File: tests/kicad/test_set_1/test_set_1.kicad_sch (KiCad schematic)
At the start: 46 parts, among them J4 Conn_01x24_Socket

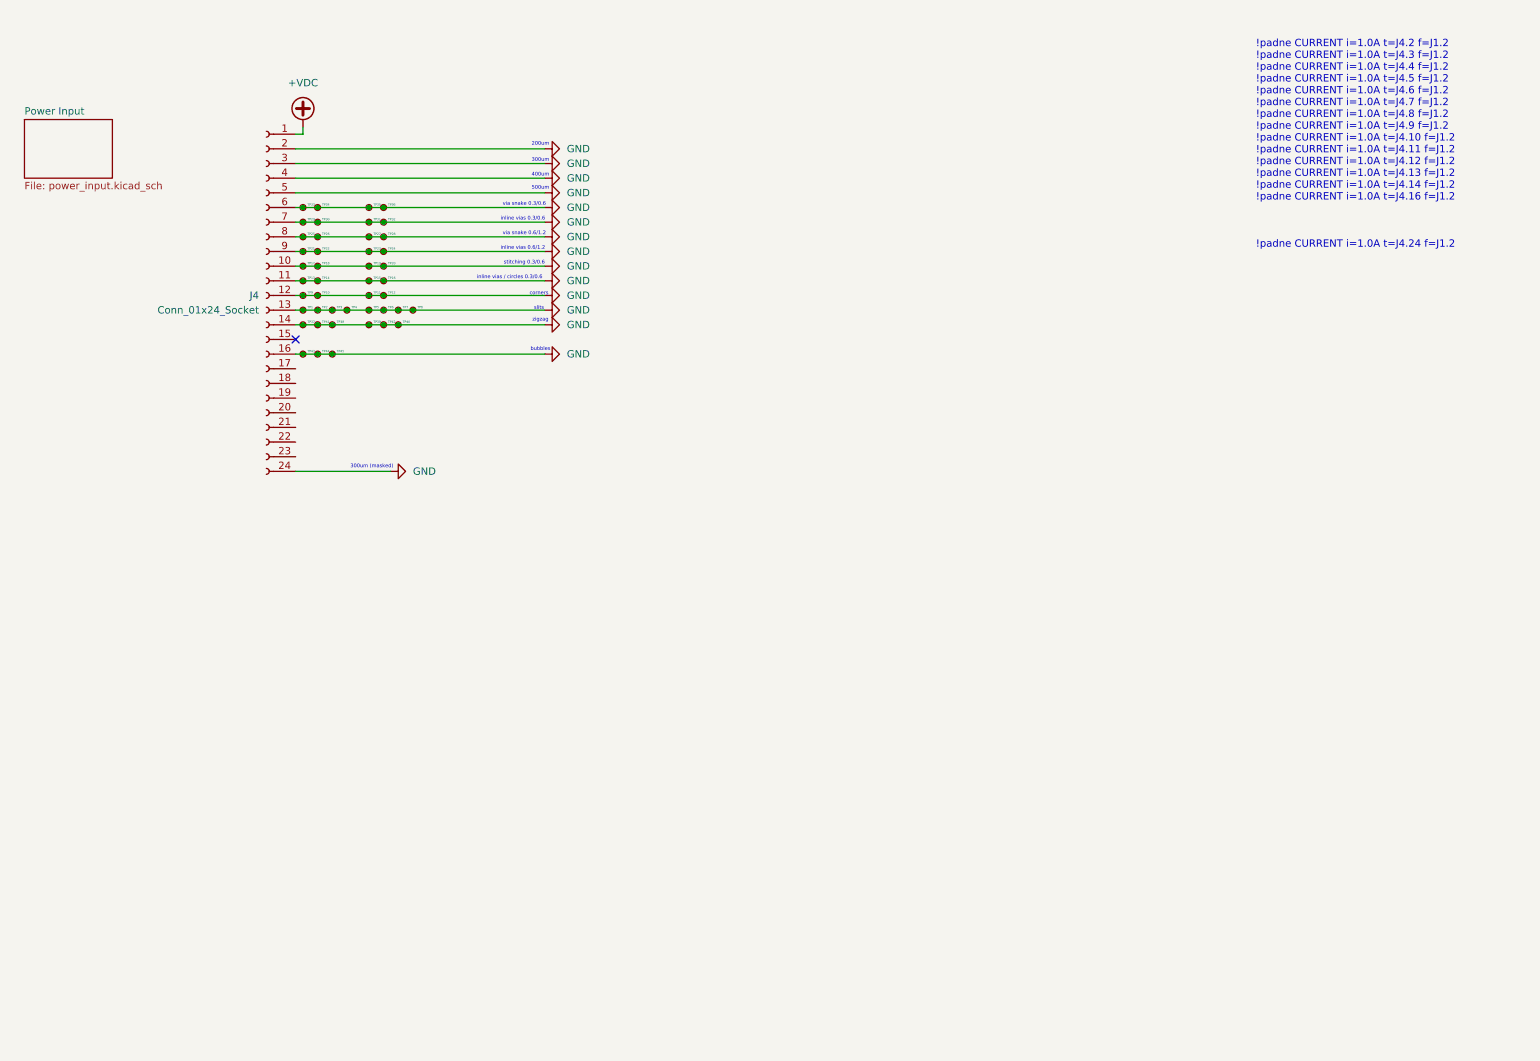
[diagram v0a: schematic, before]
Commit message: test: test_set_1 board almost finished
Gonna sleep on it a bit and then yolo order it.
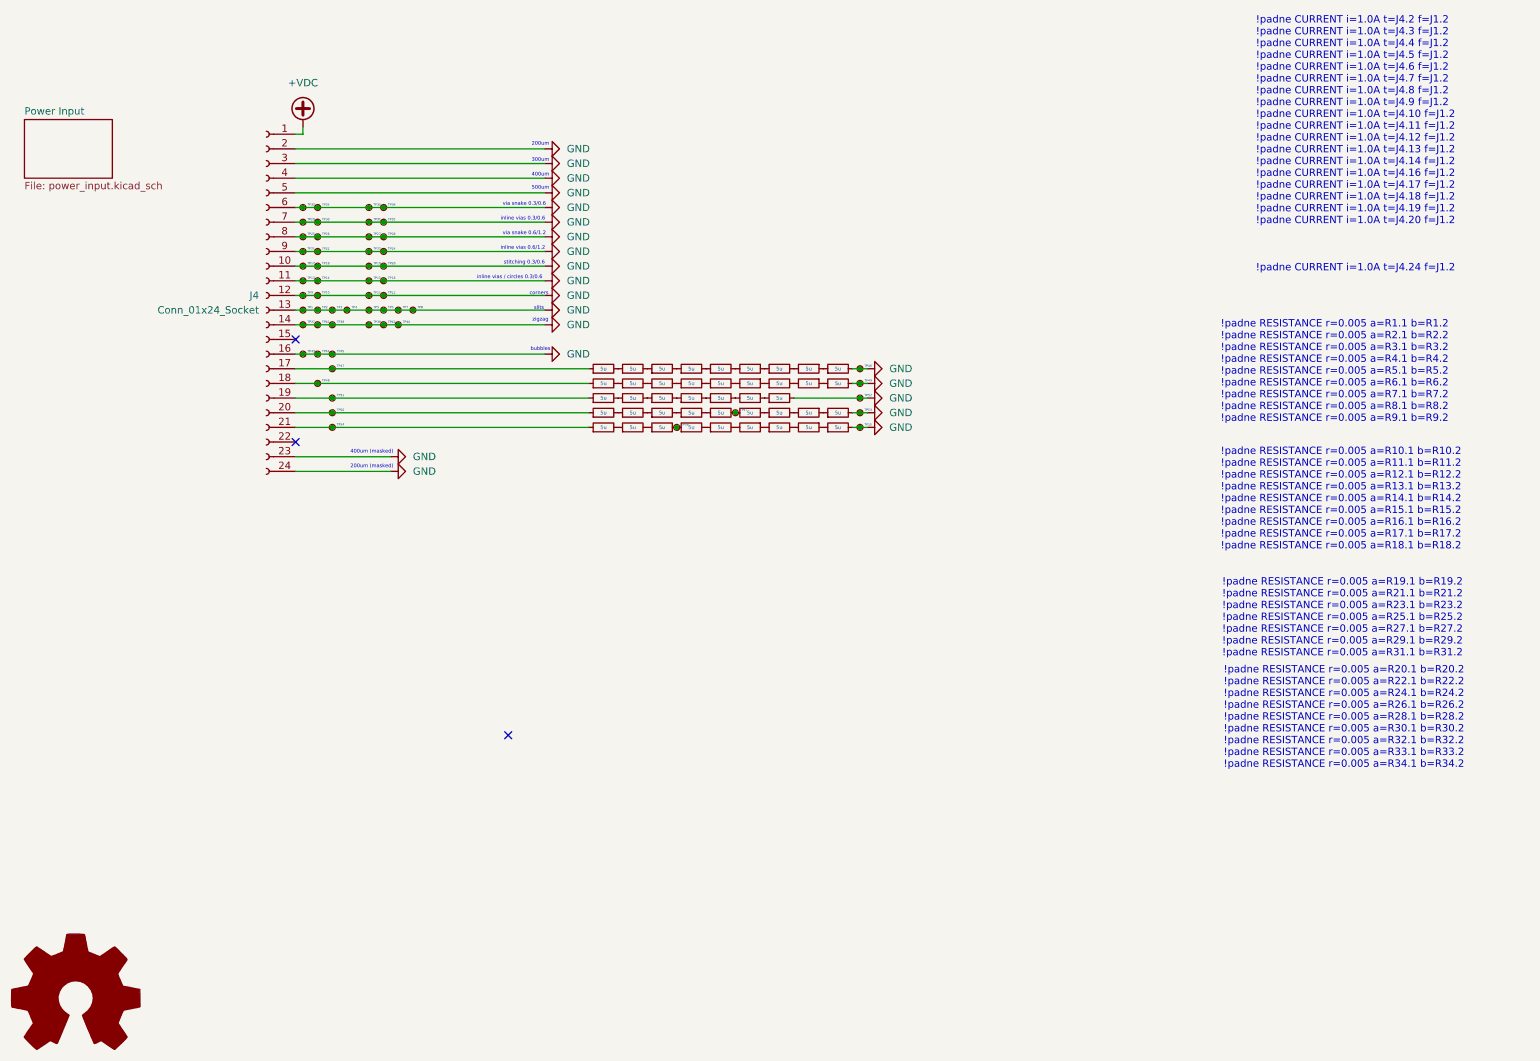
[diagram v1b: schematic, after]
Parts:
- added R1, R10, R11, R12, R13, R14, R15, R16, R17, R18, R2, R3, R4, R5, R6, R7, R8, R9: 5u, Resistor_SMD:R_1206_3216Metric, symbol Device:R_Small
- added R19, R21, R23, R25, R27, R29, R31: 5u, Resistor_SMD:R_2512_6332Metric, symbol Device:R_Small
- added R20, R22, R24, R26, R28, R30, R32, R33, R34, R35, R36, R37, R38, R39, R40, R41, R42, R43: 5u, Resistor_SMD:R_0805_2012Metric, symbol Device:R_Small
- added SYM1: Logo_Open_Hardware_Large, Symbol:OSHW-Symbol_6.7x6mm_SilkScreen, symbol Graphic:Logo_Open_Hardware_Large
- added TP46, TP47, TP48, TP49, TP50, TP51, TP52, TP53, TP54, TP55, TP56, TP57: TestPoint_Small, padne_footprints:ProbePoint, symbol Connector:TestPoint_Small
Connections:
- net GND: now also J4.23 (Pin_23), R18.2, R31.2, R34.2, R43.2, R9.2, TP46.1, TP49.1, TP52.1, TP53.1, TP55.1
- net at J4.17 (Pin_17): now also R1.1, TP47.1
- net at J4.18 (Pin_18): now also R10.1, TP48.1
- net at J4.19 (Pin_19): now also R19.1, TP51.1
- net at J4.20 (Pin_20): now also R20.1, TP50.1
- net at J4.21 (Pin_21): now also R35.1, TP54.1
- new net: R6.1, R7.1
- new net: R7.2, R8.2
- new net: R23.2, R25.1
- new net: R25.2, R27.1
- new net: R12.2, R13.1
- new net: R13.2, R14.1
- new net: R11.2, R12.1
- new net: R40.1, R41.1
- new net: R41.2, R42.2
- new net: R35.2, R36.1
- new net: R33.1, R34.1
- new net: R20.2, R22.1
- new net: R8.1, R9.1
- new net: R19.2, R21.1
- new net: R3.2, R4.1
- new net: R4.2, R5.1
- new net: R30.1, R32.1
- new net: R32.2, R33.2
- new net: R17.1, R18.1
- new net: R29.1, R31.1
- new net: R27.2, R29.2
- new net: R36.2, R37.1
- new net: R10.2, R11.1
- new net: R2.2, R3.1
- new net: R1.2, R2.1
- new net: R22.2, R24.1
- new net: R37.2, R38.1, TP56.1
- new net: R5.2, R6.2
- new net: R38.2, R39.1
- new net: R16.2, R17.2
- new net: R28.2, R30.2, TP57.1
- new net: R15.1, R16.1
- new net: R21.2, R23.1
- new net: R39.2, R40.2
- new net: R14.2, R15.2
- new net: R42.1, R43.1
- new net: R24.2, R26.1
- new net: R26.2, R28.1
- no-connect marks 1 -> 3
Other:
- note added: "!padne RESISTANCE r=0.005 a=R1.1 b=R1.2 !padne RESISTANCE r=0.005 a=R2.1 b=R2.2 !padne RESISTANCE r=0.005 a=R3.1 b=R3.2 !padne RESISTANCE r=0.005 a=R4.1 b=R4.2 !padne RESISTANCE r=0.005 a=R5.1 b=R5.2 !padne RESISTANCE r=0.005 a=R6.1 b=R6.2 !padne RESISTANCE r=0.005 a=R7.1 b=R7.2 !padne RESISTANCE r=0.005 a=R8.1 b=R8.2 !padne RESISTANCE r=0.005 a=R9.1 b=R9.2"
- note added: "!padne RESISTANCE r=0.005 a=R10.1 b=R10.2 !padne RESISTANCE r=0.005 a=R11.1 b=R11.2 !padne RESISTANCE r=0.005 a=R12.1 b=R12.2 !padne RESISTANCE r=0.005 a=R13.1 b=R13.2 !padne RESISTANCE r=0.005 a=R14.1 b=R14.2 !padne RESISTANCE r=0.005 a=R15.1 b=R15.2 !padne RESISTANCE r=0.005 a=R16.1 b=R16.2 !padne RESISTANCE r=0.005 a=R17.1 b=R17.2 !padne RESISTANCE r=0.005 a=R18.1 b=R18.2"
- note added: "!padne RESISTANCE r=0.005 a=R19.1 b=R19.2 !padne RESISTANCE r=0.005 a=R21.1 b=R21.2 !padne RESISTANCE r=0.005 a=R23.1 b=R23.2 !padne RESISTANCE r=0.005 a=R25.1 b=R25.2 !padne RESISTANCE r=0.005 a=R27.1 b=R27.2 !padne RESISTANCE r=0.005 a=R29.1 b=R29.2 !padne RESISTANCE r=0.005 a=R31.1 b=R31.2"
- note added: "!padne RESISTANCE r=0.005 a=R20.1 b=R20.2 !padne RESISTANCE r=0.005 a=R22.1 b=R22.2 !padne RESISTANCE r=0.005 a=R24.1 b=R24.2 !padne RESISTANCE r=0.005 a=R26.1 b=R26.2 !padne RESISTANCE r=0.005 a=R28.1 b=R28.2 !padne RESISTANCE r=0.005 a=R30.1 b=R30.2 !padne RESISTANCE r=0.005 a=R32.1 b=R32.2 !padne RESISTANCE r=0.005 a=R33.1 b=R33.2 !padne RESISTANCE r=0.005 a=R34.1 b=R34.2"
- note added: "200um (masked)"
- note added: "400um (masked)"
- note removed: "300um (masked)"
